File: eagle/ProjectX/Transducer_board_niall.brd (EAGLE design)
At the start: 100 x 100 mm, 104 parts, among them T1 MA40S4S, T10 MA40S4S, T100 MA40S4S, T11 MA40S4S, T12 MA40S4S, T13 MA40S4S, T14 MA40S4S, T15 MA40S4S, T16 MA40S4S, T17 MA40S4S, T18 MA40S4S, T19 MA40S4S, T2 MA40S4S, T20 MA40S4S, T21 MA40S4S, T22 MA40S4S, T23 MA40S4S, T24 MA40S4S, T25 MA40S4S, T26 MA40S4S, T27 MA40S4S, T28 MA40S4S, T29 MA40S4S, T3 MA40S4S, T30 MA40S4S, T31 MA40S4S, T32 MA40S4S, T33 MA40S4S, T34 MA40S4S, T35 MA40S4S, T36 MA40S4S, T37 MA40S4S, T38 MA40S4S, T39 MA40S4S, T4 MA40S4S, T40 MA40S4S, T41 MA40S4S, T42 MA40S4S, T43 MA40S4S, T44 MA40S4S, T45 MA40S4S, T46 MA40S4S, T47 MA40S4S, T48 MA40S4S, T49 MA40S4S, T5 MA40S4S, T50 MA40S4S, T51 MA40S4S, T52 MA40S4S, T53 MA40S4S, T54 MA40S4S, T55 MA40S4S, T56 MA40S4S, T57 MA40S4S, T58 MA40S4S, T59 MA40S4S, T6 MA40S4S, T60 MA40S4S, T61 MA40S4S, T62 MA40S4S, T63 MA40S4S, T64 MA40S4S, T65 MA40S4S, T66 MA40S4S, T67 MA40S4S, T68 MA40S4S, T69 MA40S4S, T7 MA40S4S, T70 MA40S4S, T71 MA40S4S, T72 MA40S4S, T73 MA40S4S, T74 MA40S4S, T75 MA40S4S, T76 MA40S4S, T77 MA40S4S, T78 MA40S4S, T79 MA40S4S, T8 MA40S4S, T80 MA40S4S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

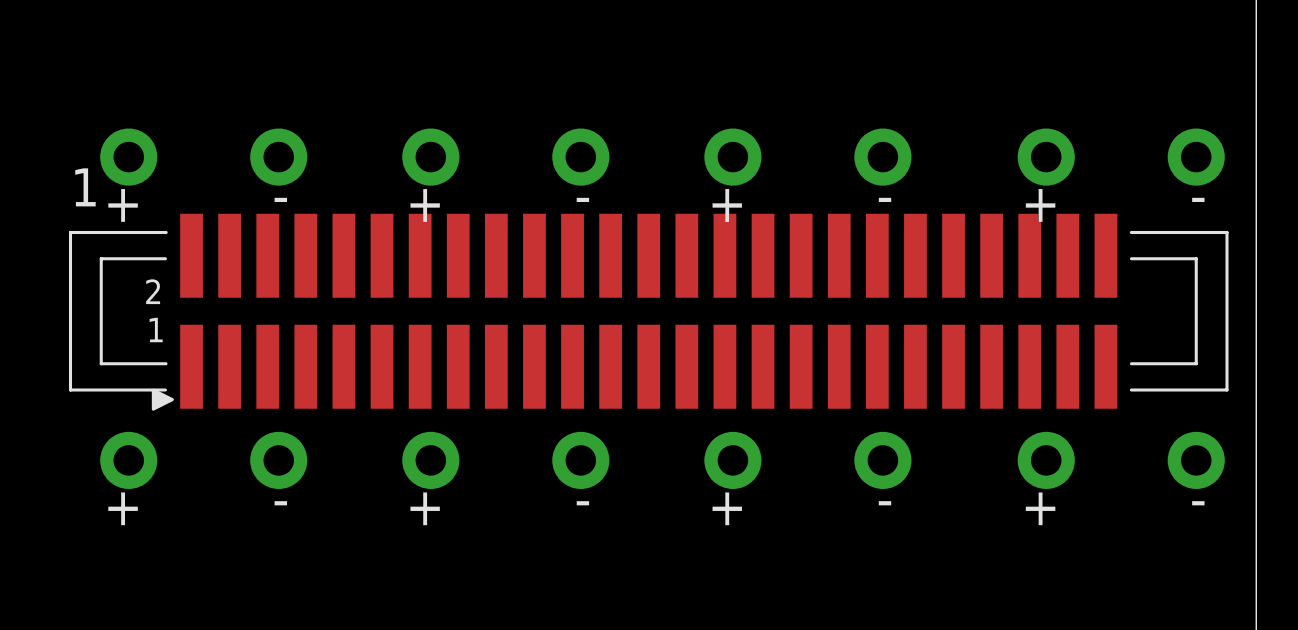
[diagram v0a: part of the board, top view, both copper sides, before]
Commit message: Niall board more work
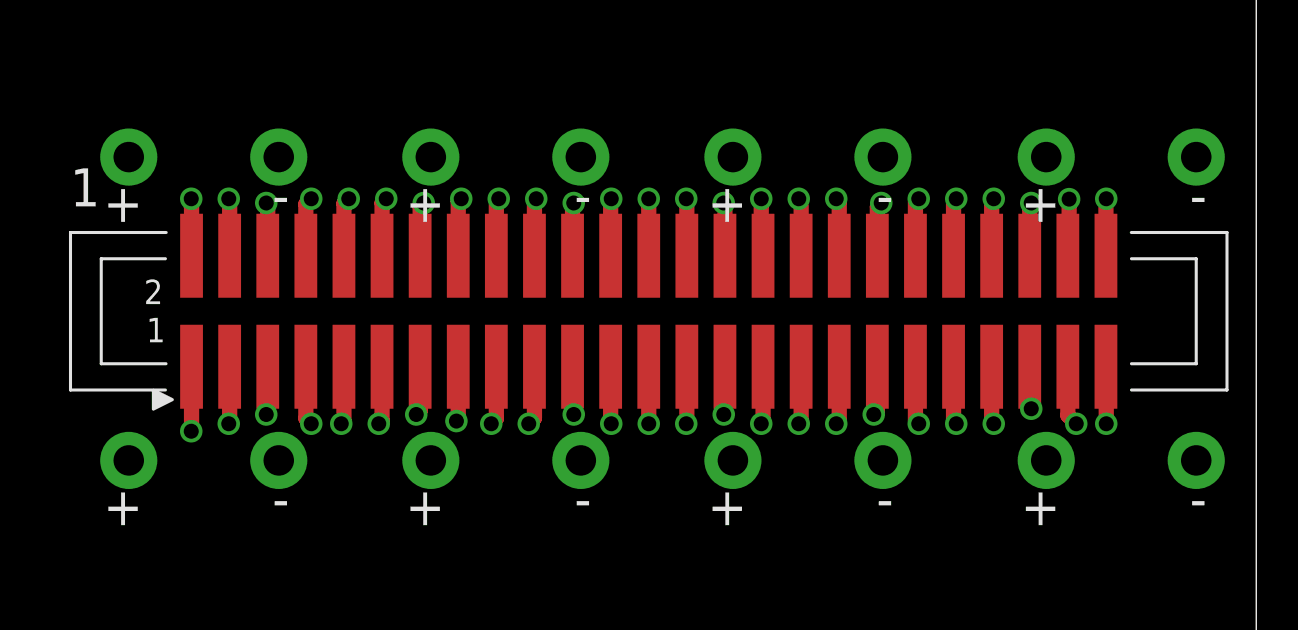
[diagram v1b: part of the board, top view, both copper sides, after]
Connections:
- new net FROM_TRANSDUCER_100: 1.50
- new net FROM_TRANSDUCER_85: 1.2
- new net FROM_TRANSDUCER_86: 1.4
- new net FROM_TRANSDUCER_87: 1.6
- new net FROM_TRANSDUCER_88: 1.8
- new net FROM_TRANSDUCER_89: 1.10
- new net FROM_TRANSDUCER_90: 1.12
- new net FROM_TRANSDUCER_91: 1.14
- new net FROM_TRANSDUCER_92: 1.16
- new net FROM_TRANSDUCER_93: 1.36
- new net FROM_TRANSDUCER_94: 1.38
- new net FROM_TRANSDUCER_95: 1.40
- new net FROM_TRANSDUCER_96: 1.42
- new net FROM_TRANSDUCER_97: 1.44
- new net FROM_TRANSDUCER_98: 1.46
- new net FROM_TRANSDUCER_99: 1.48
- new net GND: 1.18, 1.20, 1.22, 1.24, 1.26, 1.28, 1.30, 1.32, 1.34, 2.1, 2.12, 2.13, 2.16, 2.17, 2.20, 2.21, 2.24, 2.25, 2.28, 2.29, 2.32, 2.33, 2.36, 2.37, 2.4, 2.40, 2.41, 2.44, 2.45, 2.48, 2.49, 2.5, 2.8, 2.9, 3.1, 3.12, 3.13, 3.16, 3.17, 3.20, 3.21, 3.24, 3.25, 3.28, 3.29, 3.32, 3.33, 3.36, 3.37, 3.4, 3.40, 3.41, 3.44, 3.45, 3.48, 3.49, 3.5, 3.8, 3.9, 4.1, 4.12, 4.13, 4.16, 4.17, 4.20, 4.21, 4.24, 4.25, 4.28, 4.29, 4.32, 4.33, 4.36, 4.37, 4.4, 4.40, 4.41, 4.44, 4.45, 4.48, 4.49, 4.5, 4.8, 4.9
- new net N$1: T1.-
- new net N$10: T5.+
- new net N$100: T50.+
- new net N$101: T51.-
- new net N$102: T51.+
- new net N$103: T52.-
- new net N$104: T52.+
- new net N$105: T53.-
- new net N$106: T53.+
- new net N$107: T54.-
- new net N$108: T54.+
- new net N$109: T55.-
- new net N$11: T6.-
- new net N$110: T55.+
- new net N$111: T56.-
- new net N$112: T56.+
- new net N$113: T57.-
- new net N$114: T57.+
- new net N$115: T58.-
- new net N$116: T58.+
- new net N$117: T59.-
- new net N$118: T59.+
- new net N$119: T60.-
- new net N$12: T6.+
- new net N$120: T60.+
- new net N$121: T61.-
- new net N$122: T61.+
- new net N$123: T62.-
- new net N$124: T62.+
- new net N$125: T63.-
- new net N$126: T63.+
- new net N$127: T64.-
- new net N$128: T64.+
- new net N$129: T65.-
- new net N$13: T7.-
- new net N$130: T65.+
- new net N$131: T66.-
- new net N$132: T66.+
- new net N$133: T67.-
- new net N$134: T67.+
- new net N$135: T68.-
- new net N$136: T68.+
- new net N$137: T69.-
- new net N$138: T69.+
- new net N$139: T70.-
- new net N$14: T7.+
- new net N$140: T70.+
- new net N$141: T71.-
- new net N$142: T71.+
- new net N$143: T72.-
- new net N$144: T72.+
- new net N$145: T73.-
- new net N$146: T73.+
- new net N$147: T74.-
- new net N$148: T74.+
- new net N$149: T75.-
- new net N$15: T8.-
- new net N$150: T75.+
- new net N$151: T76.-
- new net N$152: T76.+
- new net N$153: T77.-
- new net N$154: T77.+
- new net N$155: T78.-
- new net N$156: T78.+
- new net N$157: T79.-
- new net N$158: T79.+
- new net N$159: T80.-
- new net N$16: T8.+
- new net N$160: T80.+
- new net N$161: T81.-
- new net N$162: T81.+
- new net N$163: T82.-
- new net N$164: T82.+
- new net N$165: T83.-
- new net N$166: T83.+
- new net N$167: T84.-
- new net N$168: T84.+
- new net N$169: T85.-
- new net N$17: T9.-
- new net N$170: T85.+
- new net N$171: T86.-
- new net N$172: T86.+
- new net N$173: T87.-
- new net N$174: T87.+
- new net N$175: T88.-
- new net N$176: T88.+
- new net N$177: T89.-
- new net N$178: T89.+
- new net N$179: T90.-
- new net N$18: T9.+
- new net N$180: T90.+
- new net N$181: T91.-
- new net N$182: T91.+
- new net N$183: T92.-
- new net N$184: T92.+
- new net N$185: T93.-
- new net N$186: T93.+
- new net N$187: T94.-
- new net N$188: T94.+
- new net N$189: T95.-
- new net N$19: T10.-
- new net N$190: T95.+
- new net N$191: T96.-
- new net N$192: T96.+
- new net N$193: T97.-
- new net N$194: T97.+
- new net N$195: T98.-
- new net N$196: T98.+
- new net N$197: T99.-
- new net N$198: T99.+
- new net N$199: T100.-
- new net N$2: T1.+
- new net N$20: T10.+
- new net N$200: T100.+
- new net N$21: T11.-
- new net N$22: T11.+
- new net N$23: T12.-
- new net N$24: T12.+
- new net N$25: T13.-
- new net N$26: T13.+
- new net N$27: T14.-
- new net N$28: T14.+
- new net N$29: T15.-
- new net N$3: T2.-
- new net N$30: T15.+
- new net N$31: T16.-
- new net N$32: T16.+
- new net N$33: T17.-
- new net N$34: T17.+
- new net N$35: T18.-
- new net N$36: T18.+
- new net N$37: T19.-
- new net N$38: T19.+
- new net N$39: T20.-
- new net N$4: T2.+
- new net N$40: T20.+
- new net N$41: T21.-
- new net N$42: T21.+
- new net N$43: T22.-
- new net N$44: T22.+
- new net N$45: T23.-
- new net N$46: T23.+
- new net N$47: T24.-
- new net N$48: T24.+
- new net N$49: T25.-
- new net N$5: T3.-
- new net N$50: T25.+
- new net N$51: T26.-
- new net N$52: T26.+
- new net N$53: T27.-
- new net N$54: T27.+
- new net N$55: T28.-
- new net N$56: T28.+
- new net N$57: T29.-
- new net N$58: T29.+
- new net N$59: T30.-
- new net N$6: T3.+
- new net N$60: T30.+
- new net N$61: T31.-
- new net N$62: T31.+
- new net N$63: T32.-
- new net N$64: T32.+
- new net N$65: T33.-
- new net N$66: T33.+
- new net N$67: T34.-
- new net N$68: T34.+
- new net N$69: T35.-
- new net N$7: T4.-
- new net N$70: T35.+
- new net N$71: T36.-
- new net N$72: T36.+
- new net N$73: T37.-
- new net N$74: T37.+
- new net N$75: T38.-
- new net N$76: T38.+
- new net N$77: T39.-
- new net N$78: T39.+
- new net N$79: T40.-
- new net N$8: T4.+
- new net N$80: T40.+
- new net N$81: T41.-
- new net N$82: T41.+
- new net N$83: T42.-
- new net N$84: T42.+
- new net N$85: T43.-
- new net N$86: T43.+
- new net N$87: T44.-
- new net N$88: T44.+
- new net N$89: T45.-
- new net N$9: T5.-
- new net N$90: T45.+
- new net N$91: T46.-
- new net N$92: T46.+
- new net N$93: T47.-
- new net N$94: T47.+
- new net N$95: T48.-
- new net N$96: T48.+
- new net N$97: T49.-
- new net N$98: T49.+
- new net N$99: T50.-
- new net TO_TRANSDUCER_100: 1.49
- new net TO_TRANSDUCER_76: 1.17
- new net TO_TRANSDUCER_77: 1.19
- new net TO_TRANSDUCER_78: 1.21
- new net TO_TRANSDUCER_79: 1.23
- new net TO_TRANSDUCER_80: 1.25
- new net TO_TRANSDUCER_81: 1.27
- new net TO_TRANSDUCER_82: 1.29
- new net TO_TRANSDUCER_83: 1.31
- new net TO_TRANSDUCER_84: 1.33
- new net TO_TRANSDUCER_85: 1.1
- new net TO_TRANSDUCER_86: 1.3
- new net TO_TRANSDUCER_87: 1.5
- new net TO_TRANSDUCER_88: 1.7
- new net TO_TRANSDUCER_89: 1.9
- new net TO_TRANSDUCER_90: 1.11
- new net TO_TRANSDUCER_91: 1.13
- new net TO_TRANSDUCER_92: 1.15
- new net TO_TRANSDUCER_93: 1.35
- new net TO_TRANSDUCER_94: 1.37
- new net TO_TRANSDUCER_95: 1.39
- new net TO_TRANSDUCER_96: 1.41
- new net TO_TRANSDUCER_97: 1.43
- new net TO_TRANSDUCER_98: 1.45
- new net TO_TRANSDUCER_99: 1.47
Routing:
- net GND: track 0.00 -> 17.0 mm, vias 0 -> 9
- net TO_TRANSDUCER_85: track 0.00 -> 2.15 mm, vias 0 -> 1
- net TO_TRANSDUCER_99: track 0.00 -> 2.02 mm, vias 0 -> 1
- net TO_TRANSDUCER_77: track 0.00 -> 1.98 mm, vias 0 -> 1
- net TO_TRANSDUCER_88: track 0.00 -> 1.97 mm, vias 0 -> 1
- net FROM_TRANSDUCER_88: track 0.00 -> 1.97 mm, vias 0 -> 1
- net TO_TRANSDUCER_76: track 0.00 -> 1.97 mm, vias 0 -> 1
- net FROM_TRANSDUCER_89: track 0.00 -> 1.97 mm, vias 0 -> 1
- net FROM_TRANSDUCER_90: track 0.00 -> 1.96 mm, vias 0 -> 1
- net TO_TRANSDUCER_95: track 0.00 -> 1.95 mm, vias 0 -> 1
- net TO_TRANSDUCER_90: track 0.00 -> 1.95 mm, vias 0 -> 1
- net FROM_TRANSDUCER_95: track 0.00 -> 1.95 mm, vias 0 -> 1
- net TO_TRANSDUCER_93: track 0.00 -> 1.94 mm, vias 0 -> 1
- net FROM_TRANSDUCER_93: track 0.00 -> 1.94 mm, vias 0 -> 1
- net FROM_TRANSDUCER_92: track 0.00 -> 1.94 mm, vias 0 -> 1
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
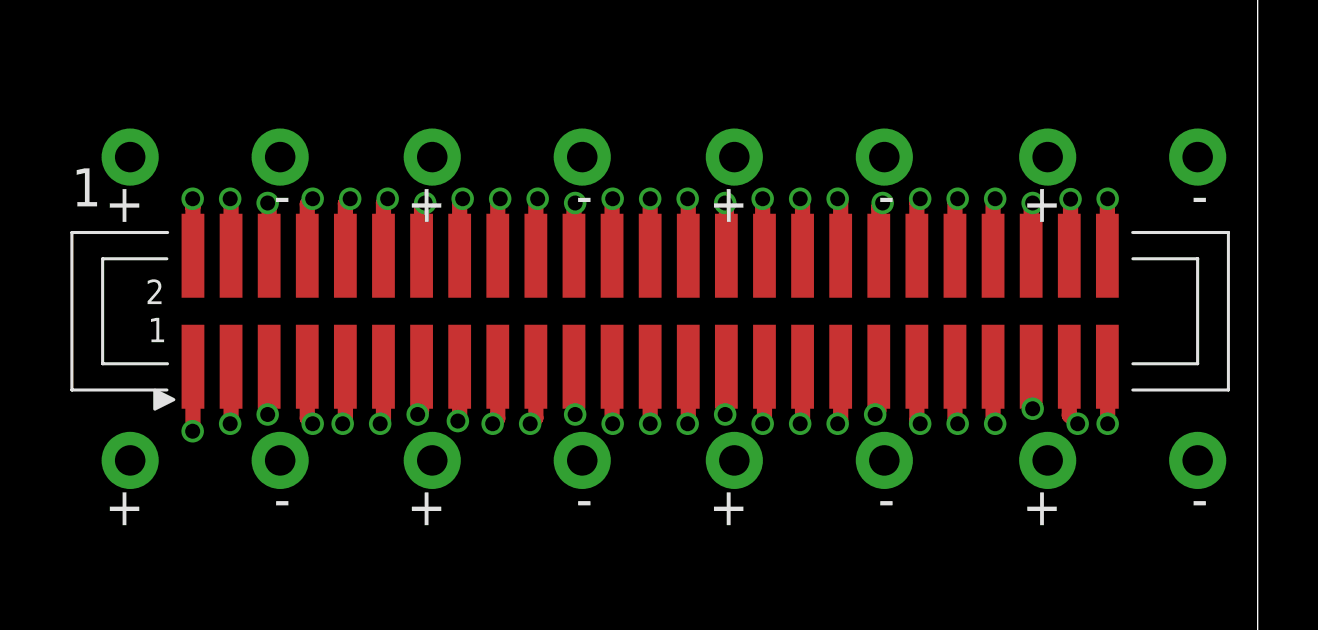
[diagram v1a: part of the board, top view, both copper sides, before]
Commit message: Transducer board start
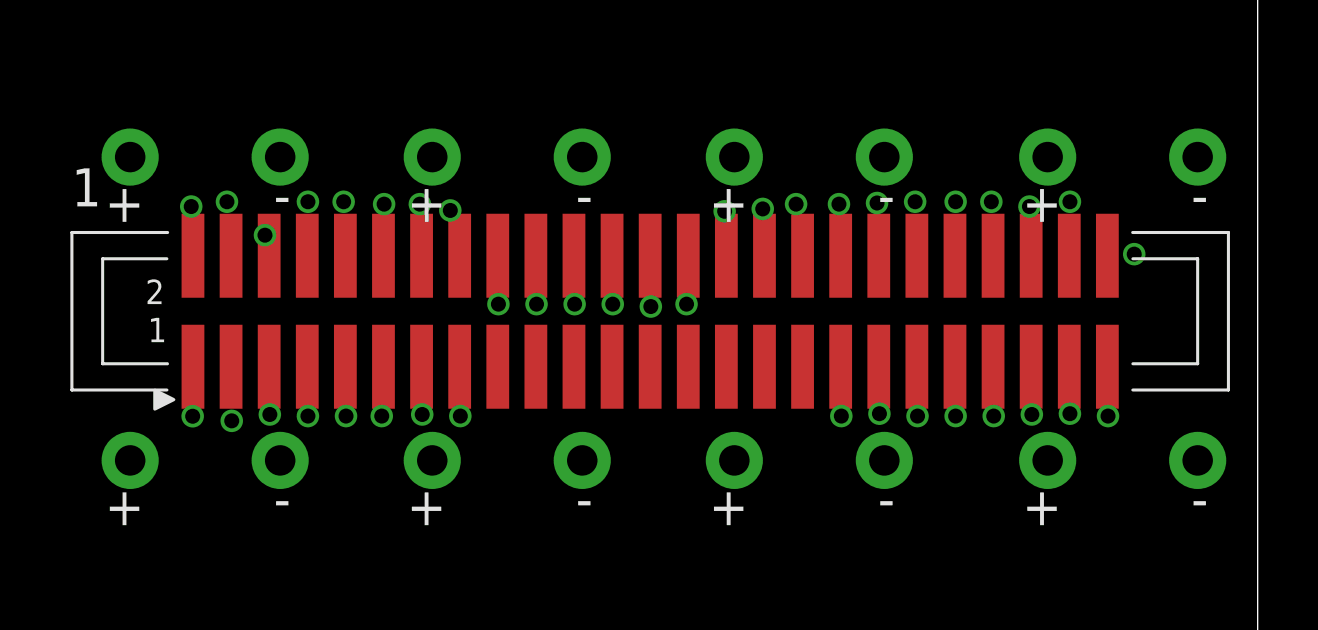
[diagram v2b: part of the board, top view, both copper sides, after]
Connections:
- net N$10 renamed TO_T_5
- net N$101 renamed FROM_T_51
- net N$102 renamed TO_T_51
- net N$107 renamed FROM_T_54
- net N$108 renamed TO_T_54
- net N$113 renamed FROM_T_57
- net N$114 renamed TO_T_57
- net N$115 renamed FROM_T_58
- net N$116 renamed TO_T_58
- net N$117 renamed FROM_T_59
- net N$118 renamed TO_T_59
- net N$121 renamed FROM_T_61
- net N$122 renamed TO_T_61
- net N$123 renamed FROM_T_62
- net N$124 renamed TO_T_62
- net N$125 renamed FROM_T_63
- net N$126 renamed TO_T_63
- net N$127 renamed FROM_T_64
- net N$128 renamed TO_T_64
- net N$129 renamed FROM_T_65
- net N$13 renamed FROM_T_7
- net N$130 renamed TO_T_65
- net N$131 renamed FROM_T_66
- net N$132 renamed TO_T_66
- net N$133 renamed FROM_T_67
- net N$134 renamed TO_T_67
- net N$139 renamed FROM_T_70
- net N$14 renamed TO_T_7
- net N$140 renamed TO_T_70
- net N$141 renamed FROM_T_71
- net N$142 renamed TO_T_71
- net N$147 renamed FROM_T_74
- net N$148 renamed TO_T_74
- net N$149 renamed FROM_T_75
- net N$15 renamed FROM_T_8
- net N$150 renamed TO_T_75
- net N$151 renamed FROM_T_76
- net N$152 renamed TO_T_76
- net N$153 renamed FROM_T_77
- net N$154 renamed TO_T_77
- net N$155 renamed FROM_T_78
- net N$156 renamed TO_T_78
- net N$159 renamed FROM_T_80
- net N$16 renamed TO_T_8
- net N$160 renamed TO_T_80
- net N$161 renamed FROM_T_81
- net N$162 renamed TO_T_81
- net N$163 renamed FROM_T_82
- net N$164 renamed TO_T_82
- net N$165 renamed FROM_T_83
- net N$166 renamed TO_T_83
- net N$167 renamed FROM_T_84
- net N$168 renamed TO_T_84
- net N$169 renamed FROM_T_85
- net N$17 renamed FROM_T_9
- net N$170 renamed TO_T_85
- net N$171 renamed FROM_T_86
- net N$172 renamed TO_T_86
- net N$173 renamed FROM_T_87
- net N$174 renamed TO_T_87
- net N$179 renamed FROM_T_90
- net N$18 renamed TO_T_9
- net N$180 renamed TO_T_90
- net N$187 renamed FROM_T_94
- net N$188 renamed TO_T_94
- net N$189 renamed FROM_T_95
- net N$190 renamed TO_T_95
- net N$193 renamed FROM_T_97
- net N$194 renamed TO_T_97
- net N$195 renamed FROM_T_98
- net N$196 renamed TO_T_98
- net N$197 renamed FROM_T_99
- net N$198 renamed TO_T_99
- net N$21 renamed FROM_T_11
- net N$22 renamed TO_T_11
- net N$23 renamed FROM_T_12
- net N$24 renamed TO_T_12
- net N$25 renamed FROM_T_13
- net N$26 renamed TO_T_13
- net N$27 renamed FROM_T_14
- net N$28 renamed TO_T_14
- net N$29 renamed FROM_T_15
- net N$3 renamed FROM_T_2
- net N$30 renamed TO_T_15
- net N$31 renamed FROM_T_16
- net N$32 renamed TO_T_16
- net N$33 renamed FROM_T_17
- net N$34 renamed TO_T_17
- net N$35 renamed FROM_T_18
- net N$36 renamed TO_T_18
- net N$37 renamed FROM_T_19
- net N$38 renamed TO_T_19
- net N$39 renamed FROM_T_20
- net N$4 renamed TO_T_2
- net N$40 renamed TO_T_20
- net N$41 renamed FROM_T_21
- net N$42 renamed TO_T_21
- net N$45 renamed FROM_T_23
- net N$46 renamed TO_T_23
- net N$47 renamed FROM_T_24
- net N$48 renamed TO_T_24
- net N$49 renamed FROM_T_25
- net N$5 renamed FROM_T_3
- net N$50 renamed TO_T_25
- net N$51 renamed FROM_T_26
- net N$52 renamed TO_T_26
- net N$53 renamed FROM_T_27
- net N$54 renamed TO_T_27
- net N$57 renamed FROM_T_29
- net N$58 renamed TO_T_29
- net N$59 renamed FROM_T_30
- net N$6 renamed TO_T_3
- net N$60 renamed TO_T_30
- net N$61 renamed FROM_T_31
- net N$62 renamed TO_T_31
- net N$63 renamed FROM_T_32
- net N$64 renamed TO_T_32
- net N$65 renamed FROM_T_33
- net N$66 renamed TO_T_33
- net N$67 renamed FROM_T_34
- net N$68 renamed TO_T_34
- net N$69 renamed FROM_T_35
- net N$7 renamed FROM_T_4
- net N$70 renamed TO_T_35
- net N$71 renamed FROM_T_36
- net N$72 renamed TO_T_36
- net N$73 renamed FROM_T_37
- net N$74 renamed TO_T_37
- net N$75 renamed FROM_T_38
- net N$76 renamed TO_T_38
- net N$77 renamed FROM_T_39
- net N$78 renamed TO_T_39
- net N$79 renamed FROM_T_40
- net N$8 renamed TO_T_4
- net N$80 renamed TO_T_40
- net N$81 renamed FROM_T_41
- net N$82 renamed TO_T_41
- net N$83 renamed FROM_T_42
- net N$84 renamed TO_T_42
- net N$85 renamed FROM_T_43
- net N$86 renamed TO_T_43
- net N$87 renamed FROM_T_44
- net N$88 renamed TO_T_44
- net N$9 renamed FROM_T_5
- net N$93 renamed FROM_T_47
- net N$94 renamed TO_T_47
- net N$95 renamed FROM_T_48
- net N$96 renamed TO_T_48
- net N$97 renamed FROM_T_49
- net N$98 renamed TO_T_49
- removed net FROM_TRANSDUCER_100: 1.50
- removed net FROM_TRANSDUCER_85: 1.2
- removed net FROM_TRANSDUCER_86: 1.4
- removed net FROM_TRANSDUCER_87: 1.6
- removed net FROM_TRANSDUCER_88: 1.8
- removed net FROM_TRANSDUCER_89: 1.10
- removed net FROM_TRANSDUCER_90: 1.12
- removed net FROM_TRANSDUCER_91: 1.14
- removed net FROM_TRANSDUCER_92: 1.16
- removed net FROM_TRANSDUCER_93: 1.36
- removed net FROM_TRANSDUCER_94: 1.38
- removed net FROM_TRANSDUCER_95: 1.40
- removed net FROM_TRANSDUCER_96: 1.42
- removed net FROM_TRANSDUCER_97: 1.44
- removed net FROM_TRANSDUCER_98: 1.46
- removed net FROM_TRANSDUCER_99: 1.48
- removed net GND: 1.18, 1.20, 1.22, 1.24, 1.26, 1.28, 1.30, 1.32, 1.34, 2.1, 2.12, 2.13, 2.16, 2.17, 2.20, 2.21, 2.24, 2.25, 2.28, 2.29, 2.32, 2.33, 2.36, 2.37, 2.4, 2.40, 2.41, 2.44, 2.45, 2.48, 2.49, 2.5, 2.8, 2.9, 3.1, 3.12, 3.13, 3.16, 3.17, 3.20, 3.21, 3.24, 3.25, 3.28, 3.29, 3.32, 3.33, 3.36, 3.37, 3.4, 3.40, 3.41, 3.44, 3.45, 3.48, 3.49, 3.5, 3.8, 3.9, 4.1, 4.12, 4.13, 4.16, 4.17, 4.20, 4.21, 4.24, 4.25, 4.28, 4.29, 4.32, 4.33, 4.36, 4.37, 4.4, 4.40, 4.41, 4.44, 4.45, 4.48, 4.49, 4.5, 4.8, 4.9
- removed net N$1: T1.-
- removed net N$100: T50.+
- removed net N$103: T52.-
- removed net N$104: T52.+
- removed net N$105: T53.-
- removed net N$106: T53.+
- removed net N$109: T55.-
- removed net N$11: T6.-
- removed net N$110: T55.+
- removed net N$111: T56.-
- removed net N$112: T56.+
- removed net N$119: T60.-
- removed net N$12: T6.+
- removed net N$120: T60.+
- removed net N$135: T68.-
- removed net N$136: T68.+
- removed net N$137: T69.-
- removed net N$138: T69.+
- removed net N$143: T72.-
- removed net N$144: T72.+
- removed net N$145: T73.-
- removed net N$146: T73.+
- removed net N$157: T79.-
- removed net N$158: T79.+
- removed net N$175: T88.-
- removed net N$176: T88.+
- removed net N$177: T89.-
- removed net N$178: T89.+
- removed net N$181: T91.-
- removed net N$182: T91.+
- removed net N$183: T92.-
- removed net N$184: T92.+
- removed net N$185: T93.-
- removed net N$186: T93.+
- removed net N$19: T10.-
- removed net N$191: T96.-
- removed net N$192: T96.+
- removed net N$199: T100.-
- removed net N$2: T1.+
- removed net N$20: T10.+
- removed net N$200: T100.+
- removed net N$43: T22.-
- removed net N$44: T22.+
- removed net N$55: T28.-
- removed net N$56: T28.+
- removed net N$89: T45.-
- removed net N$90: T45.+
- removed net N$91: T46.-
- removed net N$92: T46.+
- removed net N$99: T50.-
- removed net TO_TRANSDUCER_100: 1.49
- removed net TO_TRANSDUCER_76: 1.17
- removed net TO_TRANSDUCER_77: 1.19
- removed net TO_TRANSDUCER_78: 1.21
- removed net TO_TRANSDUCER_79: 1.23
- removed net TO_TRANSDUCER_80: 1.25
- removed net TO_TRANSDUCER_81: 1.27
- removed net TO_TRANSDUCER_82: 1.29
- removed net TO_TRANSDUCER_83: 1.31
- removed net TO_TRANSDUCER_84: 1.33
- removed net TO_TRANSDUCER_85: 1.1
- removed net TO_TRANSDUCER_86: 1.3
- removed net TO_TRANSDUCER_87: 1.5
- removed net TO_TRANSDUCER_88: 1.7
- removed net TO_TRANSDUCER_89: 1.9
- removed net TO_TRANSDUCER_90: 1.11
- removed net TO_TRANSDUCER_91: 1.13
- removed net TO_TRANSDUCER_92: 1.15
- removed net TO_TRANSDUCER_93: 1.35
- removed net TO_TRANSDUCER_94: 1.37
- removed net TO_TRANSDUCER_95: 1.39
- removed net TO_TRANSDUCER_96: 1.41
- removed net TO_TRANSDUCER_97: 1.43
- removed net TO_TRANSDUCER_98: 1.45
- removed net TO_TRANSDUCER_99: 1.47
- new net FROM_T_1: 1.2, T1.-
- new net FROM_T_10: 1.6, T10.-
- new net FROM_T_100: 1.48, T100.-
- new net FROM_T_22: 1.40, T22.-
- new net FROM_T_28: 1.12, T28.-
- new net FROM_T_45: 1.14, T45.-
- new net FROM_T_46: 1.16, T46.-
- new net FROM_T_50: 1.8, T50.-
- new net FROM_T_52: 1.22, T52.-
- new net FROM_T_53: 1.24, T53.-
- new net FROM_T_55: 1.36, T55.-
- new net FROM_T_56: 1.38, T56.-
- new net FROM_T_6: 1.4, T6.-
- new net FROM_T_60: 1.10, T60.-
- new net FROM_T_68: 1.20, T68.-
- new net FROM_T_69: 1.26, T69.-
- new net FROM_T_72: 1.42, T72.-
- new net FROM_T_73: 1.18, T73.-
- new net FROM_T_79: 1.44, T79.-
- new net FROM_T_88: 1.30, T88.-
- new net FROM_T_89: 1.28, T89.-
- new net FROM_T_91: 1.50, T91.-
- new net FROM_T_92: 1.32, T92.-
- new net FROM_T_93: 1.34, T93.-
- new net FROM_T_96: 1.46, T96.-
- new net TO_T_1: 1.1, T1.+
- new net TO_T_10: 1.5, T10.+
- new net TO_T_100: 1.47, T100.+
- new net TO_T_22: 1.39, T22.+
- new net TO_T_28: 1.11, T28.+
- new net TO_T_45: 1.13, T45.+
- new net TO_T_46: 1.15, T46.+
- new net TO_T_50: 1.7, T50.+
- new net TO_T_52: 1.21, T52.+
- new net TO_T_53: 1.23, T53.+
- new net TO_T_55: 1.35, T55.+
- new net TO_T_56: 1.37, T56.+
- new net TO_T_6: 1.3, T6.+
- new net TO_T_60: 1.9, T60.+
- new net TO_T_68: 1.19, T68.+
- new net TO_T_69: 1.25, T69.+
- new net TO_T_72: 1.41, T72.+
- new net TO_T_73: 1.17, T73.+
- new net TO_T_79: 1.43, T79.+
- new net TO_T_88: 1.29, T88.+
- new net TO_T_89: 1.27, T89.+
- new net TO_T_91: 1.49, T91.+
- new net TO_T_92: 1.31, T92.+
- new net TO_T_93: 1.33, T93.+
- new net TO_T_96: 1.45, T96.+
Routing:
- net GND: track 17.0 -> 0.00 mm, vias 9 -> 0
- net TO_TRANSDUCER_85: track 2.15 -> 0.00 mm, vias 1 -> 0
- net TO_TRANSDUCER_99: track 2.02 -> 0.00 mm, vias 1 -> 0
- net TO_TRANSDUCER_77: track 1.98 -> 0.00 mm, vias 1 -> 0
- net TO_TRANSDUCER_88: track 1.97 -> 0.00 mm, vias 1 -> 0
- net FROM_TRANSDUCER_88: track 1.97 -> 0.00 mm, vias 1 -> 0
- net TO_TRANSDUCER_76: track 1.97 -> 0.00 mm, vias 1 -> 0
- net FROM_TRANSDUCER_89: track 1.97 -> 0.00 mm, vias 1 -> 0
- net FROM_TRANSDUCER_90: track 1.96 -> 0.00 mm, vias 1 -> 0
- net TO_TRANSDUCER_95: track 1.95 -> 0.00 mm, vias 1 -> 0
- net TO_TRANSDUCER_90: track 1.95 -> 0.00 mm, vias 1 -> 0
- net FROM_TRANSDUCER_95: track 1.95 -> 0.00 mm, vias 1 -> 0
- net TO_TRANSDUCER_93: track 1.94 -> 0.00 mm, vias 1 -> 0
- net FROM_TRANSDUCER_93: track 1.94 -> 0.00 mm, vias 1 -> 0
- net FROM_TRANSDUCER_92: track 1.94 -> 0.00 mm, vias 1 -> 0
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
